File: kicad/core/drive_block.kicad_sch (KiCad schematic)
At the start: 8 parts, among them J20 N_HSn, J21 N_LSn, Q10 FDS8958A, U20 TC4427A

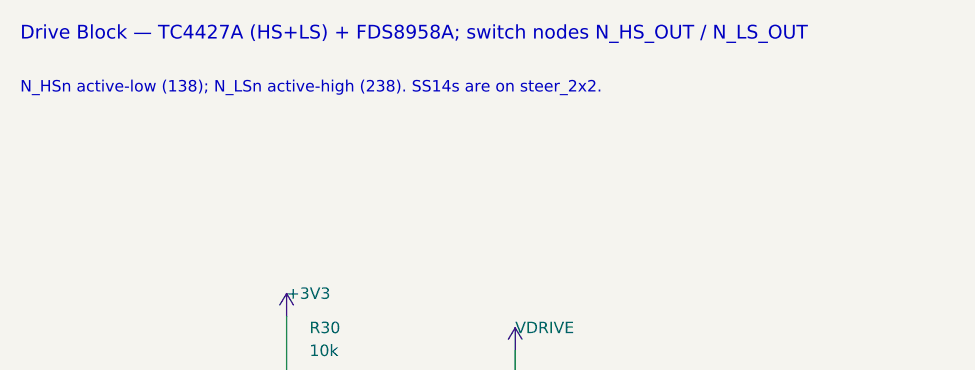
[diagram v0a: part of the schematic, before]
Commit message: Scaled to 64x64 and paying heavy due. We can learn if we have to... I guess.
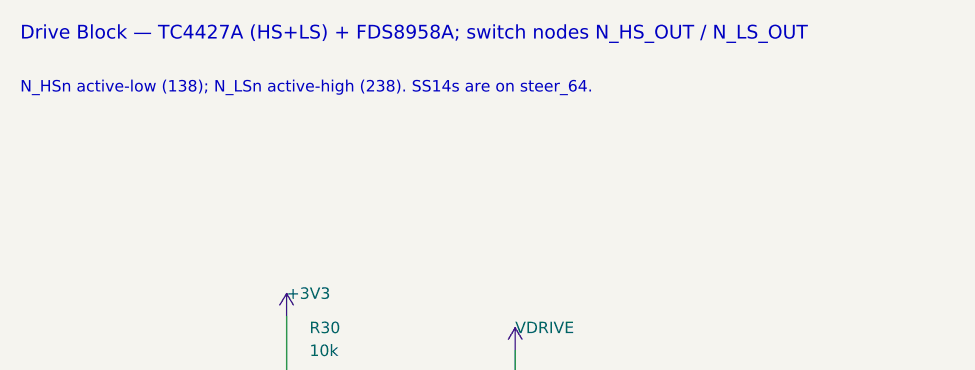
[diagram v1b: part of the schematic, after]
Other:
- note added: "N_HSn active-low (138); N_LSn active-high (238). SS14s are on steer_64."
- note removed: "N_HSn active-low (138); N_LSn active-high (238). SS14s are on steer_2x2."
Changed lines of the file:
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@@
 		(effects (font (size 1.524 1.524)) (justify left))
 	)
-	(text "N_HSn active-low (138); N_LSn active-high (238). SS14s are on steer_2x2."
+	(text "N_HSn active-low (138); N_LSn active-high (238). SS14s are on steer_64."
 		(exclude_from_sim no)
 		(at 20 18 0)
